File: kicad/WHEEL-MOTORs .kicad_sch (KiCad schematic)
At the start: 28 parts, among them J12 WHEEL-MOTOR-RIGHT, J13 WHEEL-MOTOR-LEFT, U14 DRV8870DDAR, U15 DRV8870DDAR

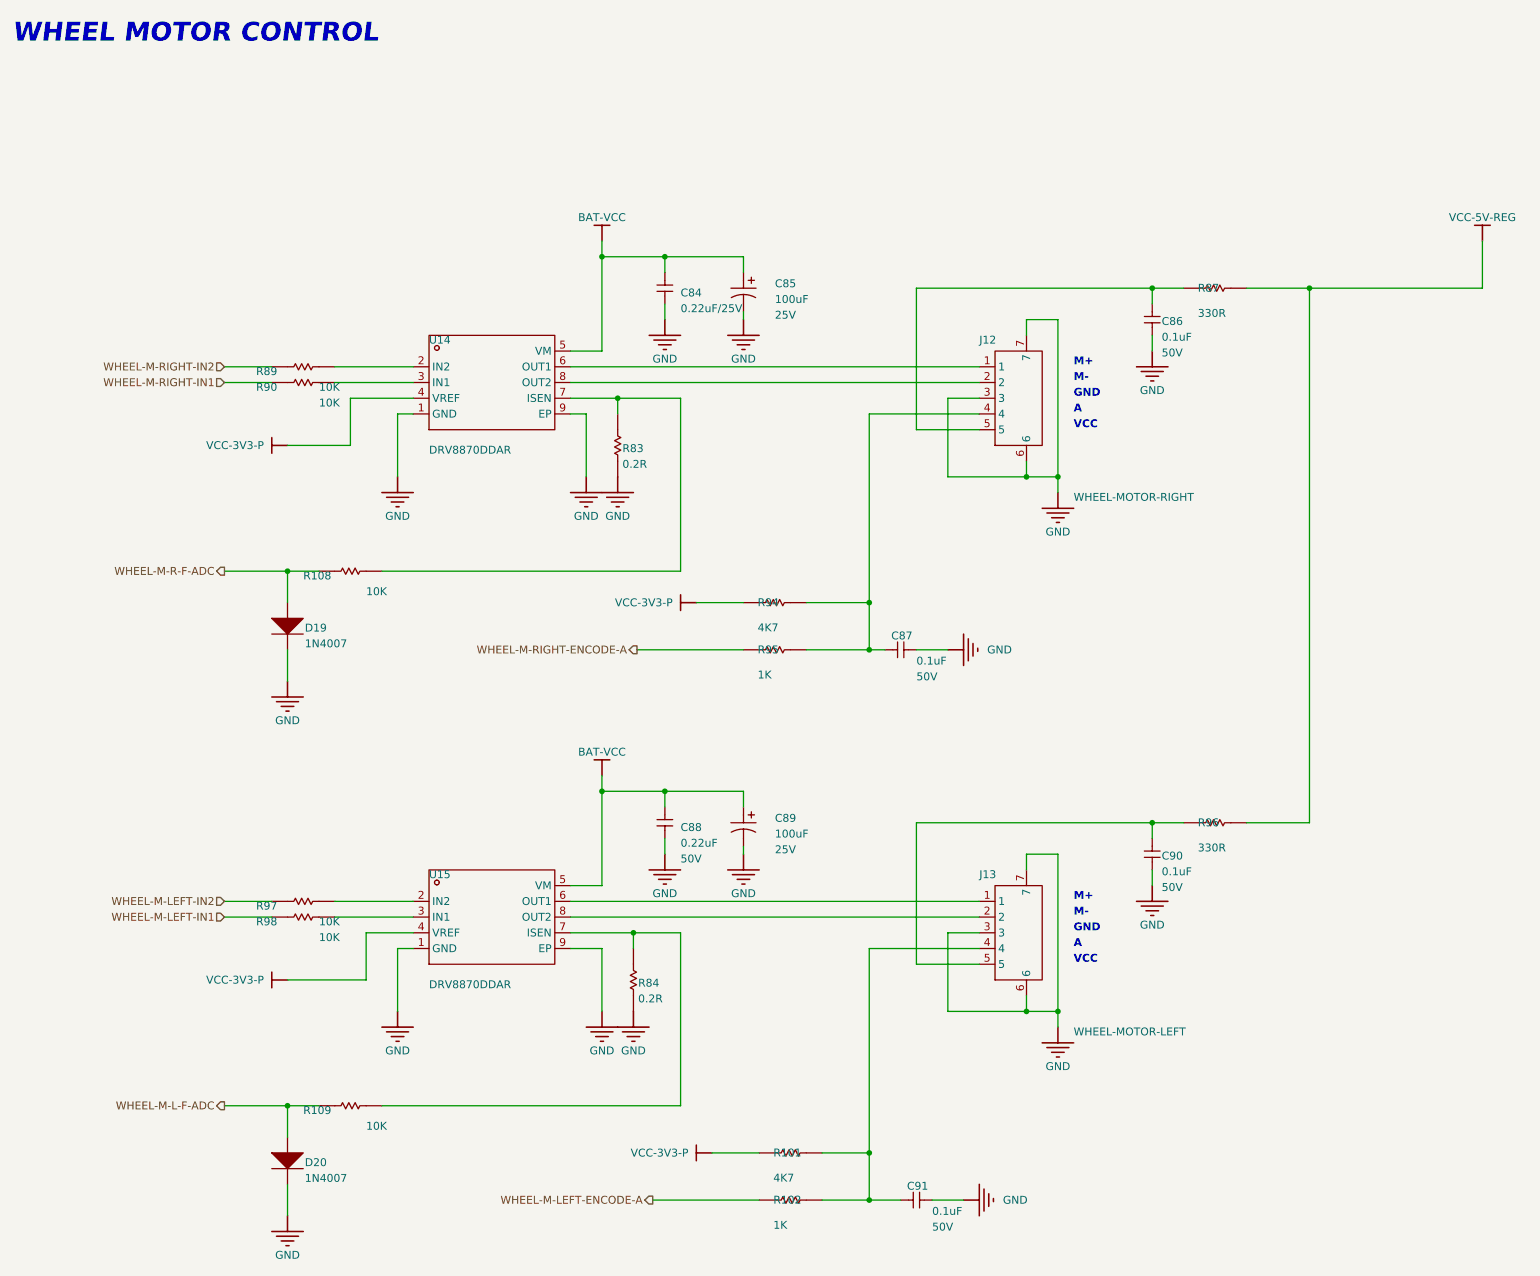
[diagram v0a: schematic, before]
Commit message: STM32G473VCT6
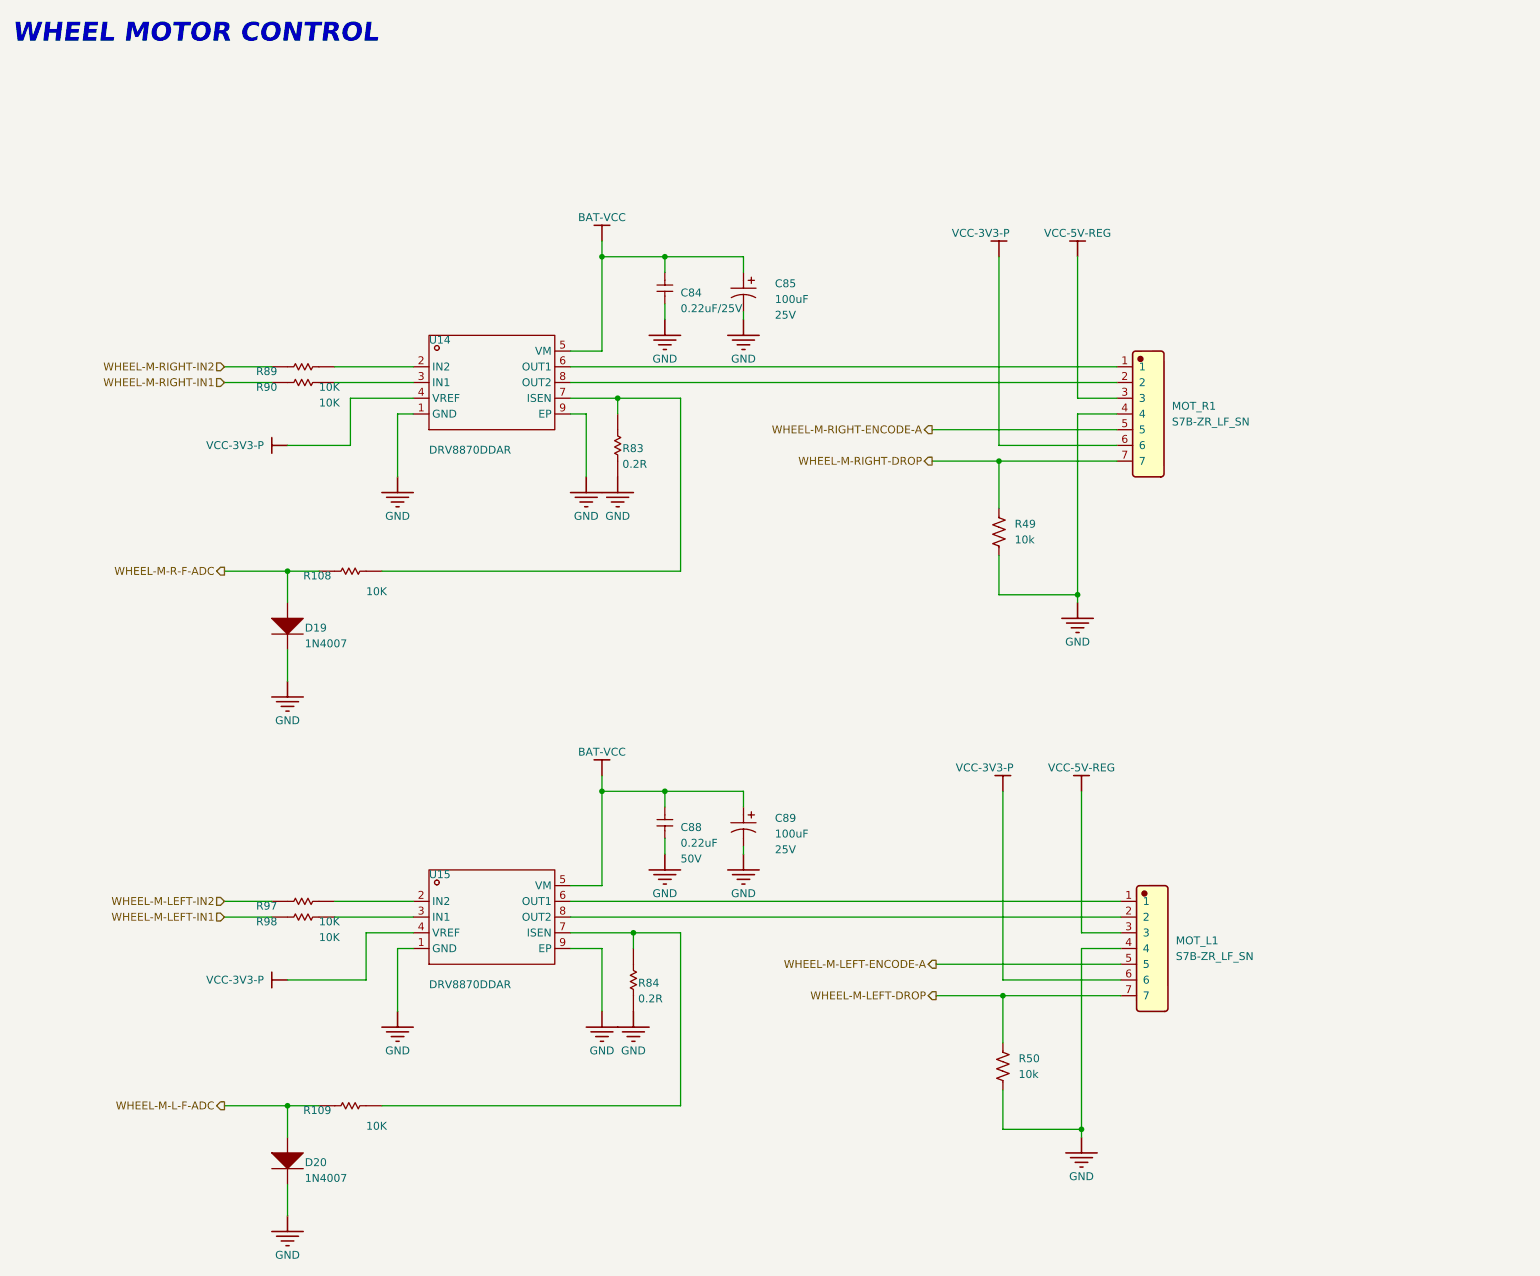
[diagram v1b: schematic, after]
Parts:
- removed C86, C90: 0.1uF, Capacitor_SMD:C_0603_1608Metric, symbol DesignLibrary:WHEEL MOTOR_3_Capacitor-1_DesignLibrary.SchLib
- removed C87, C91: 0.1uF, Capacitor_SMD:C_0603_1608Metric, symbol DesignLibrary:WHEEL MOTOR_2_Capacitor-1_DesignLibrary.SchLib
- removed J12: WHEEL-MOTOR-RIGHT, oomwoo_altium:CONN-SMD_5P-P1.50_ZX-ZH1.5-5PWT, symbol DesignLibrary:WHEEL MOTOR_0_HDRx5_DesignLibrary.SchLib
- removed J13: WHEEL-MOTOR-LEFT, oomwoo_altium:CONN-SMD_5P-P1.50_ZX-ZH1.5-5PWT, symbol DesignLibrary:WHEEL MOTOR_0_HDRx5_DesignLibrary.SchLib
- removed R101, R94: 4K7, Resistor_SMD:R_0603_1608Metric, symbol DesignLibrary:WHEEL MOTOR_0_Resistor-1_DesignLibrary.SchLib
- removed R102, R95: 1K, Resistor_SMD:R_0603_1608Metric, symbol DesignLibrary:WHEEL MOTOR_0_Resistor-1_DesignLibrary.SchLib
- removed R87, R96: 330R, Resistor_SMD:R_0603_1608Metric, symbol DesignLibrary:WHEEL MOTOR_0_Resistor-1_DesignLibrary.SchLib
- added MOT_L1, MOT_R1: S7B-ZR_LF_SN, JLCImport:S7B-ZR_LF_SN, symbol JLCImport:S7B-ZR_LF_SN
- added R49, R50: 10k, symbol Device:R_US
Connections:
- net GND: now also MOT_L1.4, MOT_R1.4, R49.2, R50.2
- net VCC-3V3-P: now also MOT_L1.6, MOT_R1.6
- net VCC-5V-REG: now also MOT_L1.3, MOT_R1.3
- net WHEEL-M-LEFT-ENCODE-A: now also MOT_L1.5
- net WHEEL-M-RIGHT-ENCODE-A: now also MOT_R1.5
- net at U14.6 (OUT1): now also MOT_R1.1
- net at U14.8 (OUT2): now also MOT_R1.2
- net at U15.6 (OUT1): now also MOT_L1.1
- net at U15.8 (OUT2): now also MOT_L1.2
- new net WHEEL-M-LEFT-DROP: MOT_L1.7, R50.1
- new net WHEEL-M-RIGHT-DROP: MOT_R1.7, R49.1
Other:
- note removed: "A"
- note removed: "GND"
- note removed: "M+"
- note removed: "M-"
- note removed: "VCC"
